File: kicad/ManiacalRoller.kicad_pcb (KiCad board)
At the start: 2 copper layers, 69.5 x 71 mm, 37 parts, among them CON1 AVR-ISP-6, IC1 ATMEGA328P-P, Q1 Q_NPN_EBC, Q2 Q_NPN_EBC, SW1 BTN_coin, SW2 BTN_d4, SW3 BTN_d6, SW4 BTN_d8, SW5 BTN_d10, SW6 BTN_d12, SW7 BTN_d20, SW8 BTN_d100, U1 74LS148

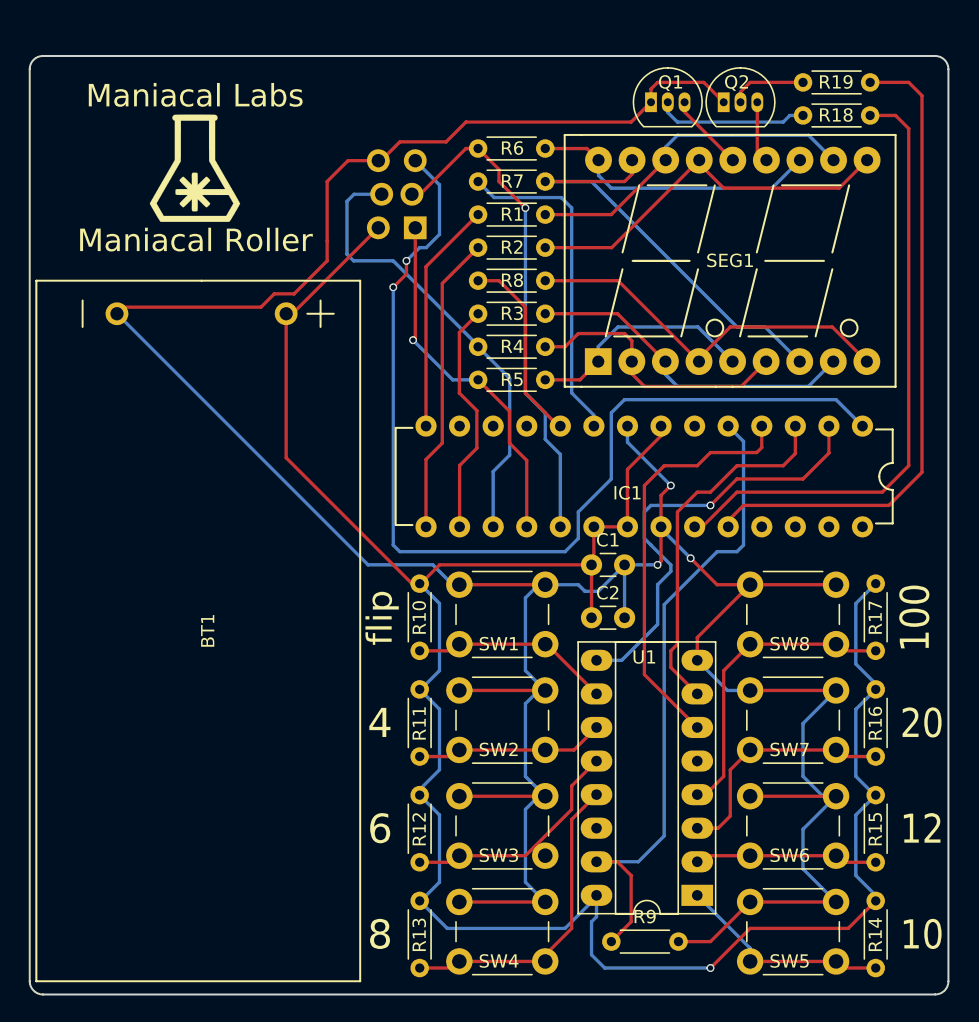
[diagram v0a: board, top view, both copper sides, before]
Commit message: Bat Hlder on back
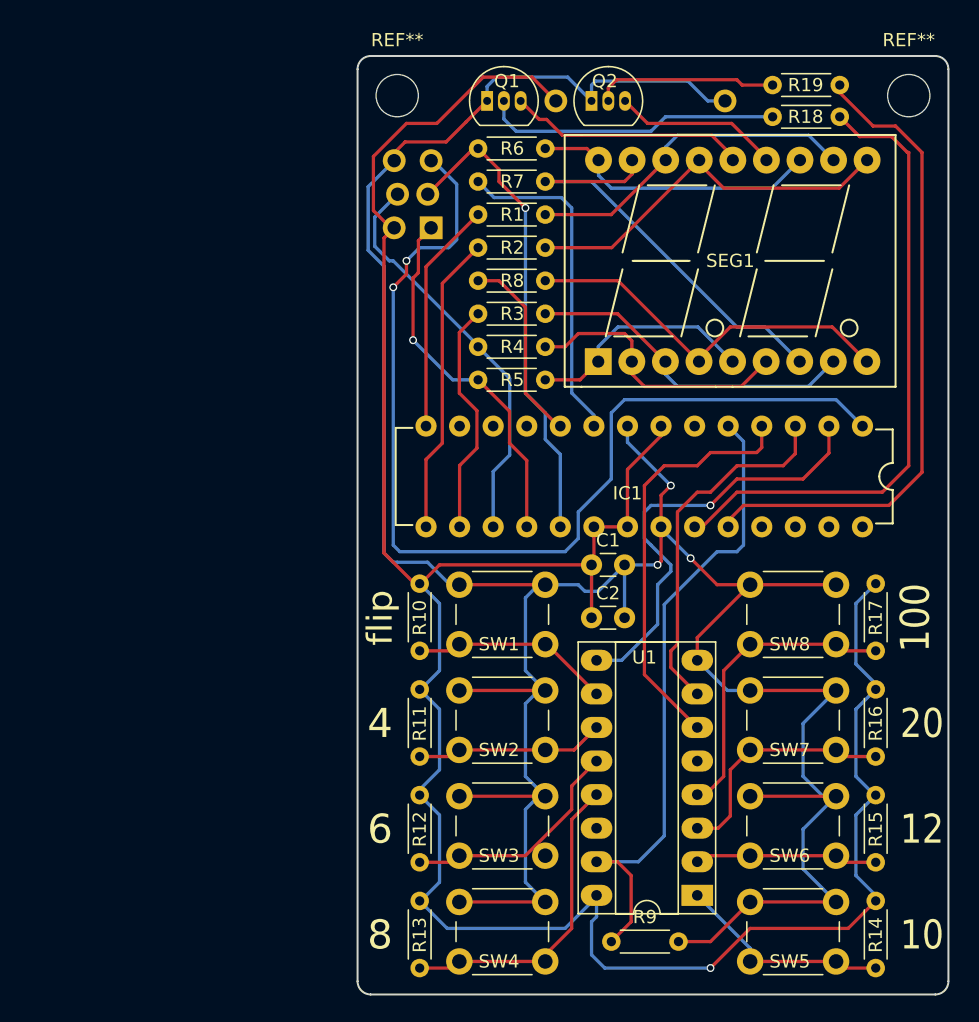
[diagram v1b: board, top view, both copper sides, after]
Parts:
- added REF**: MountingHole_3.2mm_M3, Mounting_Holes:MountingHole_3.2mm_M3, F.Cu at (154.0, 44.5)
- added REF**: MountingHole_3.2mm_M3, Mounting_Holes:MountingHole_3.2mm_M3, F.Cu at (115.3, 44.5)
- BT1, G***: moved to B.Cu
- moved G*** 49.8 mm to (149.1, 58.3), turned to 180 degrees
- moved BT1 36.9 mm to (133.7, 68.9)
- moved Q1 12.4 mm to (122.1, 44.9)
- moved Q2 10.0 mm to (130.0, 44.9)
- moved R19 2.31 mm to (143.7, 43.7)
- moved R18 2.30 mm to (143.7, 46.1)
- moved CON1 1.20 mm to (115.2, 54.5)
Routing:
- net GND: track 247.0 -> 224.3 mm
- net VBATT: track 166.0 -> 183.2 mm
- net D1: track 5.89 -> 18.1 mm
- net Net-(Q1-Pad2): track 11.5 -> 22.5 mm
- net Net-(Q2-Pad2): track 5.80 -> 13.8 mm
- net D2: track 4.67 -> 12.6 mm
- net MOSI: track 34.8 -> 30.8 mm
- net RST: track 77.0 -> 78.6 mm
- net TENS: track 46.9 -> 48.2 mm
- net SCK: track 37.6 -> 36.4 mm
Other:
- board size 69.5 x 71 mm -> 44.7 x 71 mm
